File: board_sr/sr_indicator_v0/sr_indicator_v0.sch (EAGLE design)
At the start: 11 parts

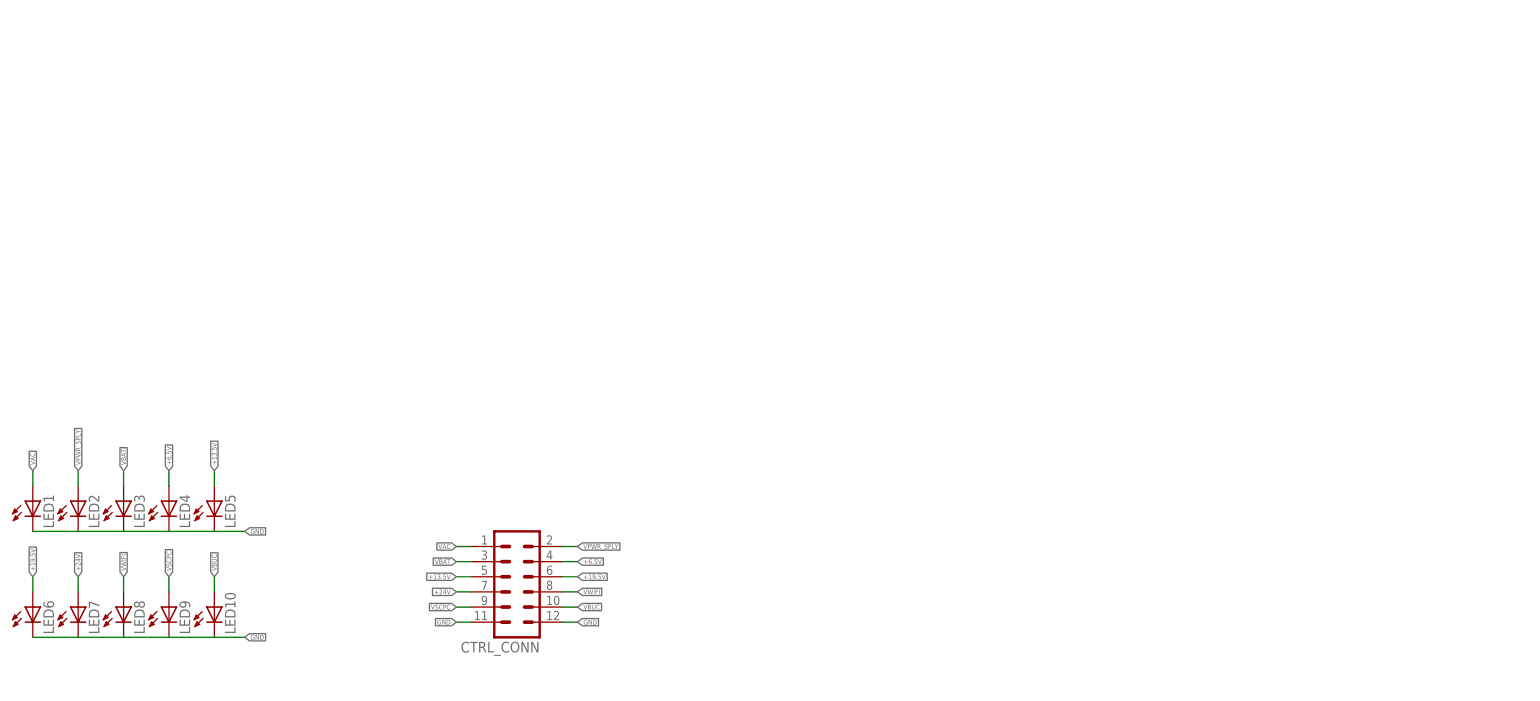
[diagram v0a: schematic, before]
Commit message: Finish routing
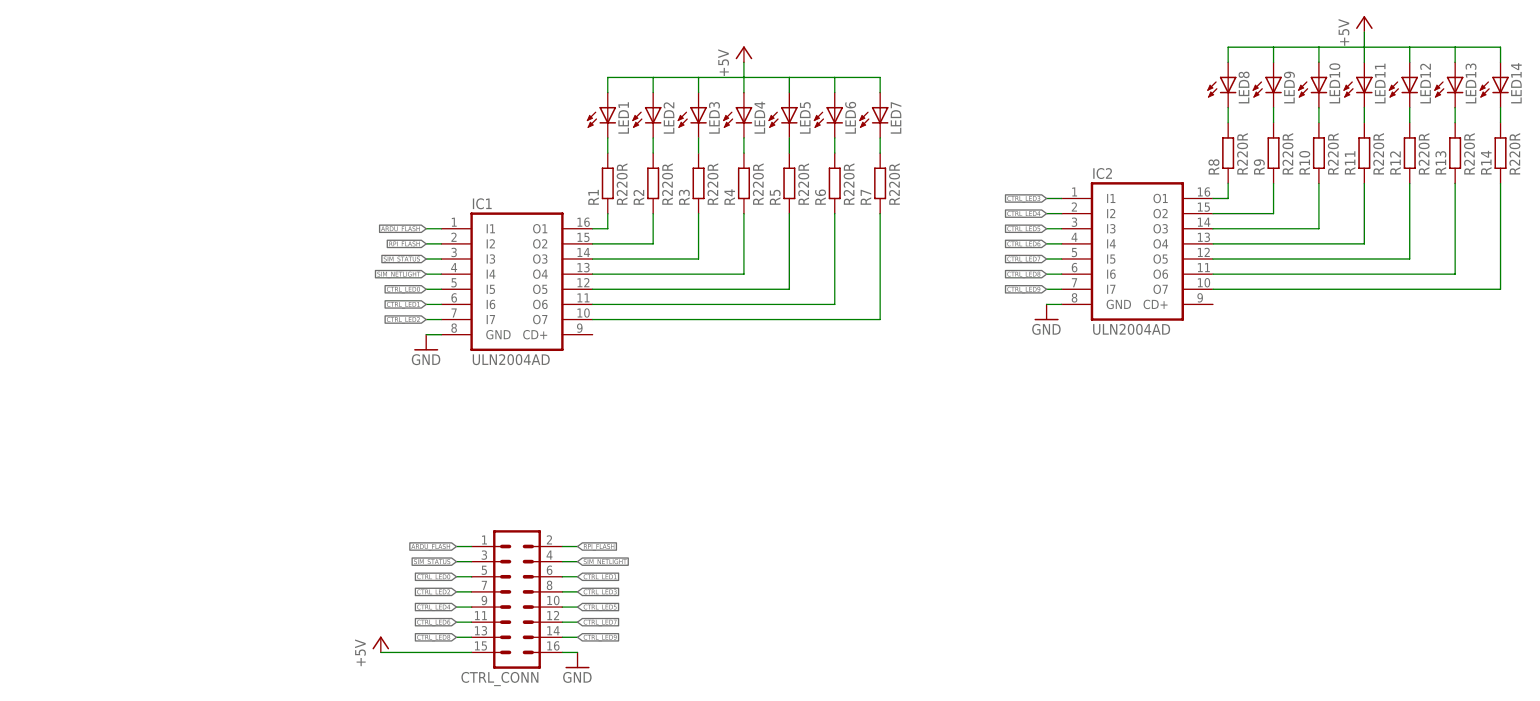
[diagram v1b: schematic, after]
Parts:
- added IC1, IC2: ULN2004AD, uln-udn:ULN2004AD
- added LED11, LED12, LED13, LED14: (no value), adafruit:LED3MM
- added R1, R10, R11, R12, R13, R14, R2, R3, R4, R5, R6, R7, R8, R9: R220R, resistor:R-EU_M0805
- CTRL_CONN: device con-lstb:MA06-2 -> con-lstb:MA08-2
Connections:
- removed net +13.5V: CTRL_CONN.5, LED5.A
- removed net +19.5V: CTRL_CONN.6, LED6.A
- removed net +24V: CTRL_CONN.7, LED7.A
- removed net +6.5V: CTRL_CONN.4, LED4.A
- removed net VAC: CTRL_CONN.1, LED1.A
- removed net VBAT: CTRL_CONN.3, LED3.A
- removed net VBUC: CTRL_CONN.10, LED10.A
- removed net VPWR_SPLY: CTRL_CONN.2, LED2.A
- removed net VSCPC: CTRL_CONN.9, LED9.A
- removed net VWIFI: CTRL_CONN.8, LED8.A
- new net +5V: CTRL_CONN.15, LED1.A, LED10.A, LED11.A, LED12.A, LED13.A, LED14.A, LED2.A, LED3.A, LED4.A, LED5.A, LED6.A, LED7.A, LED8.A, LED9.A
- new net ARDU_FLASH: CTRL_CONN.1, IC1.I1
- new net CTRL_LED0: CTRL_CONN.5, IC1.I5
- new net CTRL_LED1: CTRL_CONN.6, IC1.I6
- new net CTRL_LED2: CTRL_CONN.7, IC1.I7
- new net CTRL_LED3: CTRL_CONN.8, IC2.I1
- new net CTRL_LED4: CTRL_CONN.9, IC2.I2
- new net CTRL_LED5: CTRL_CONN.10, IC2.I3
- new net CTRL_LED6: CTRL_CONN.11, IC2.I4
- new net CTRL_LED7: CTRL_CONN.12, IC2.I5
- new net CTRL_LED8: CTRL_CONN.13, IC2.I6
- new net CTRL_LED9: CTRL_CONN.14, IC2.I7
- new net N$1: IC1.O1, R1.1
- new net N$10: LED3.C, R3.2
- new net N$11: LED4.C, R4.2
- new net N$12: LED5.C, R5.2
- new net N$13: LED6.C, R6.2
- new net N$14: LED7.C, R7.2
- new net N$15: IC2.O1, R8.1
- new net N$16: IC2.O2, R9.1
- new net N$17: IC2.O3, R10.1
- new net N$18: IC2.O4, R11.1
- new net N$19: IC2.O5, R12.1
- new net N$2: IC1.O2, R2.1
- new net N$20: IC2.O6, R13.1
- new net N$21: IC2.O7, R14.1
- new net N$22: LED8.C, R8.2
- new net N$23: LED9.C, R9.2
- new net N$24: LED10.C, R10.2
- new net N$25: LED11.C, R11.2
- new net N$26: LED12.C, R12.2
- new net N$27: LED13.C, R13.2
- new net N$28: LED14.C, R14.2
- new net N$3: IC1.O3, R3.1
- new net N$4: IC1.O4, R4.1
- new net N$5: IC1.O5, R5.1
- new net N$6: IC1.O6, R6.1
- new net N$7: IC1.O7, R7.1
- new net N$8: LED1.C, R1.2
- new net N$9: LED2.C, R2.2
- new net RPI_FLASH: CTRL_CONN.2, IC1.I2
- new net SIM_NETLIGHT: CTRL_CONN.4, IC1.I4
- new net SIM_STATUS: CTRL_CONN.3, IC1.I3
- net GND: now also CTRL_CONN.16, IC1.GND, IC2.GND; no longer CTRL_CONN.11, CTRL_CONN.12, LED1.C, LED10.C, LED2.C, LED3.C, LED4.C, LED5.C, LED6.C, LED7.C, LED8.C, LED9.C
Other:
- moved on the sheet: LED1, LED10, LED2, LED3, LED4, LED5, LED6, LED7, LED8, LED9
